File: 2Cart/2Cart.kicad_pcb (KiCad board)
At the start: 2 copper layers, 90 x 56.8 mm, 11 parts, among them J1 CommanderX16Expansion Alt, U1 SST39SF040, U2 74HCT00, U3 74HCT138, U4 AS6C4008-55PCN

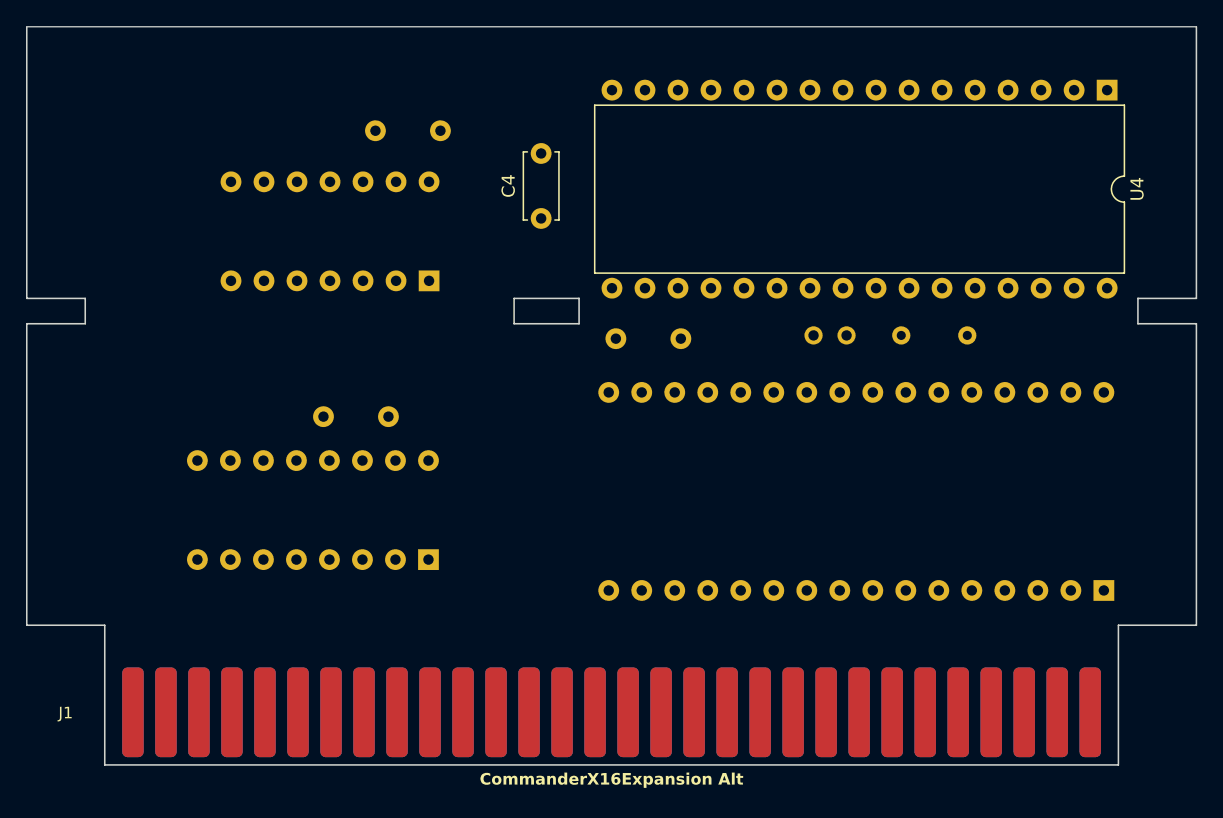
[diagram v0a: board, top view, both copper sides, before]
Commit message: Flip the board
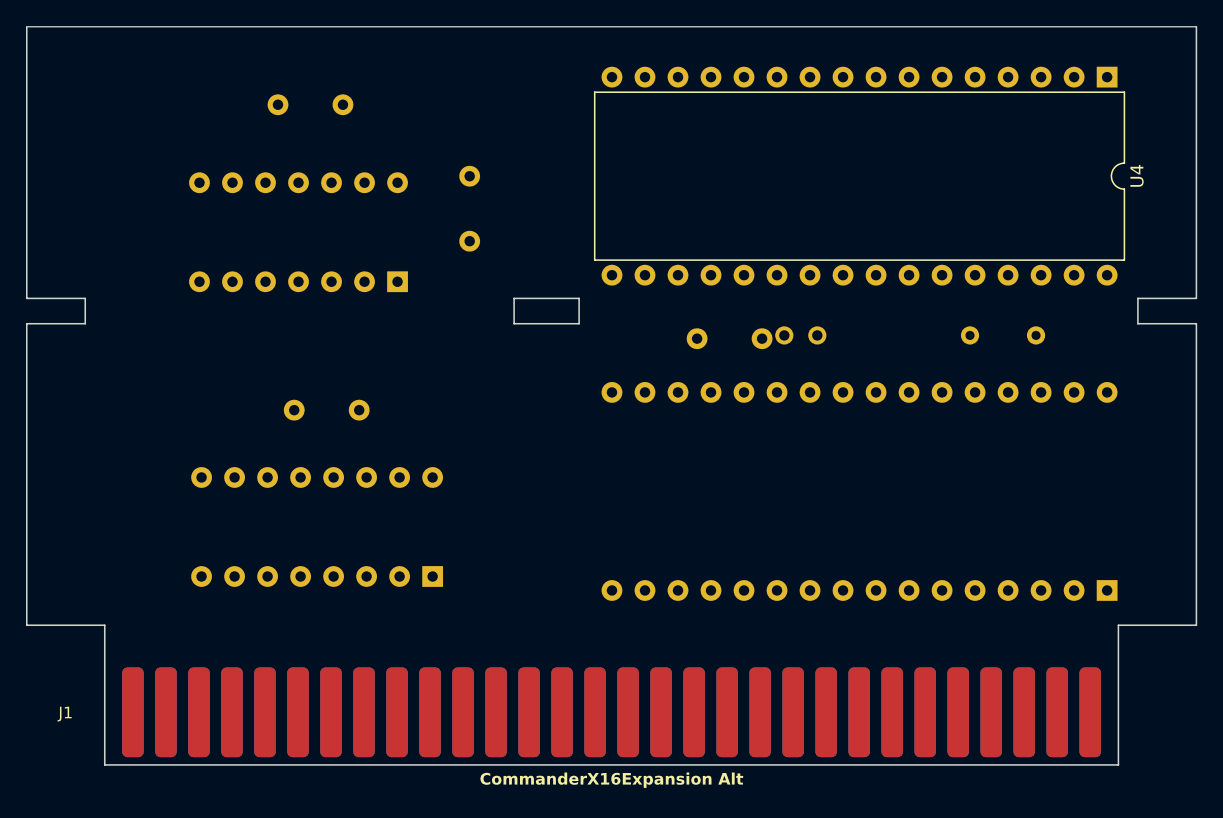
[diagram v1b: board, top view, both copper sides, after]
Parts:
- C1, C2, C3: value C -> 100nF
- C4: value C -> 100nF; moved to B.Cu
- U1: value SST39SF040 -> SST39SF040 (ROM)
- U4: value AS6C4008-55PCN -> AS6C4008 (RAM)
- moved C3 7.76 mm to (71.8, 84.0)
- moved C1 6.25 mm to (99.0, 102.0)
- moved C4 5.77 mm to (81.5, 94.5)
- moved R1 5.29 mm to (120.0, 101.8)
- moved U2 2.43 mm to (76.0, 97.6)
- moved C2 2.30 mm to (68.0, 107.5)
- moved JP1 2.25 mm to (108.2, 101.8)
- moved U3 1.34 mm to (78.7, 120.3)
- moved U4 1.00 mm to (130.6, 81.9)
- moved U1 0.25 mm to (130.6, 121.4)
